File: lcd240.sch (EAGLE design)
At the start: 27 parts, among them IC1 CAT4238TD-GT3

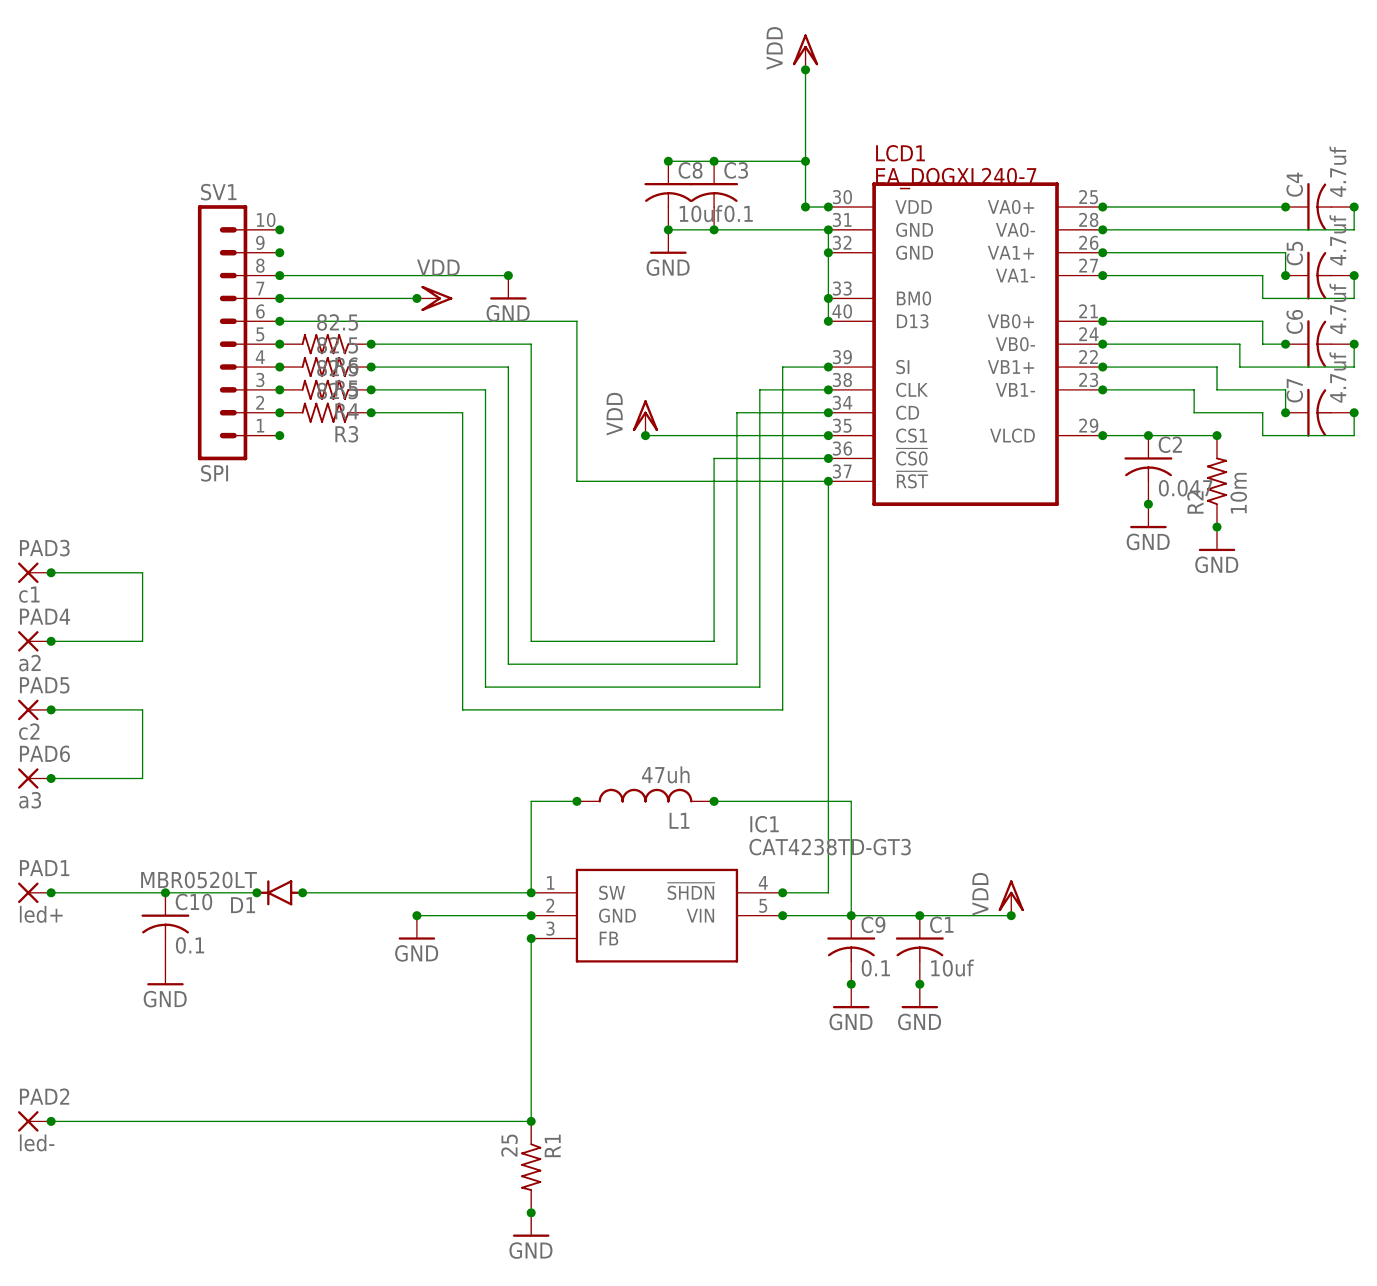
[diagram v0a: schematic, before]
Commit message: up
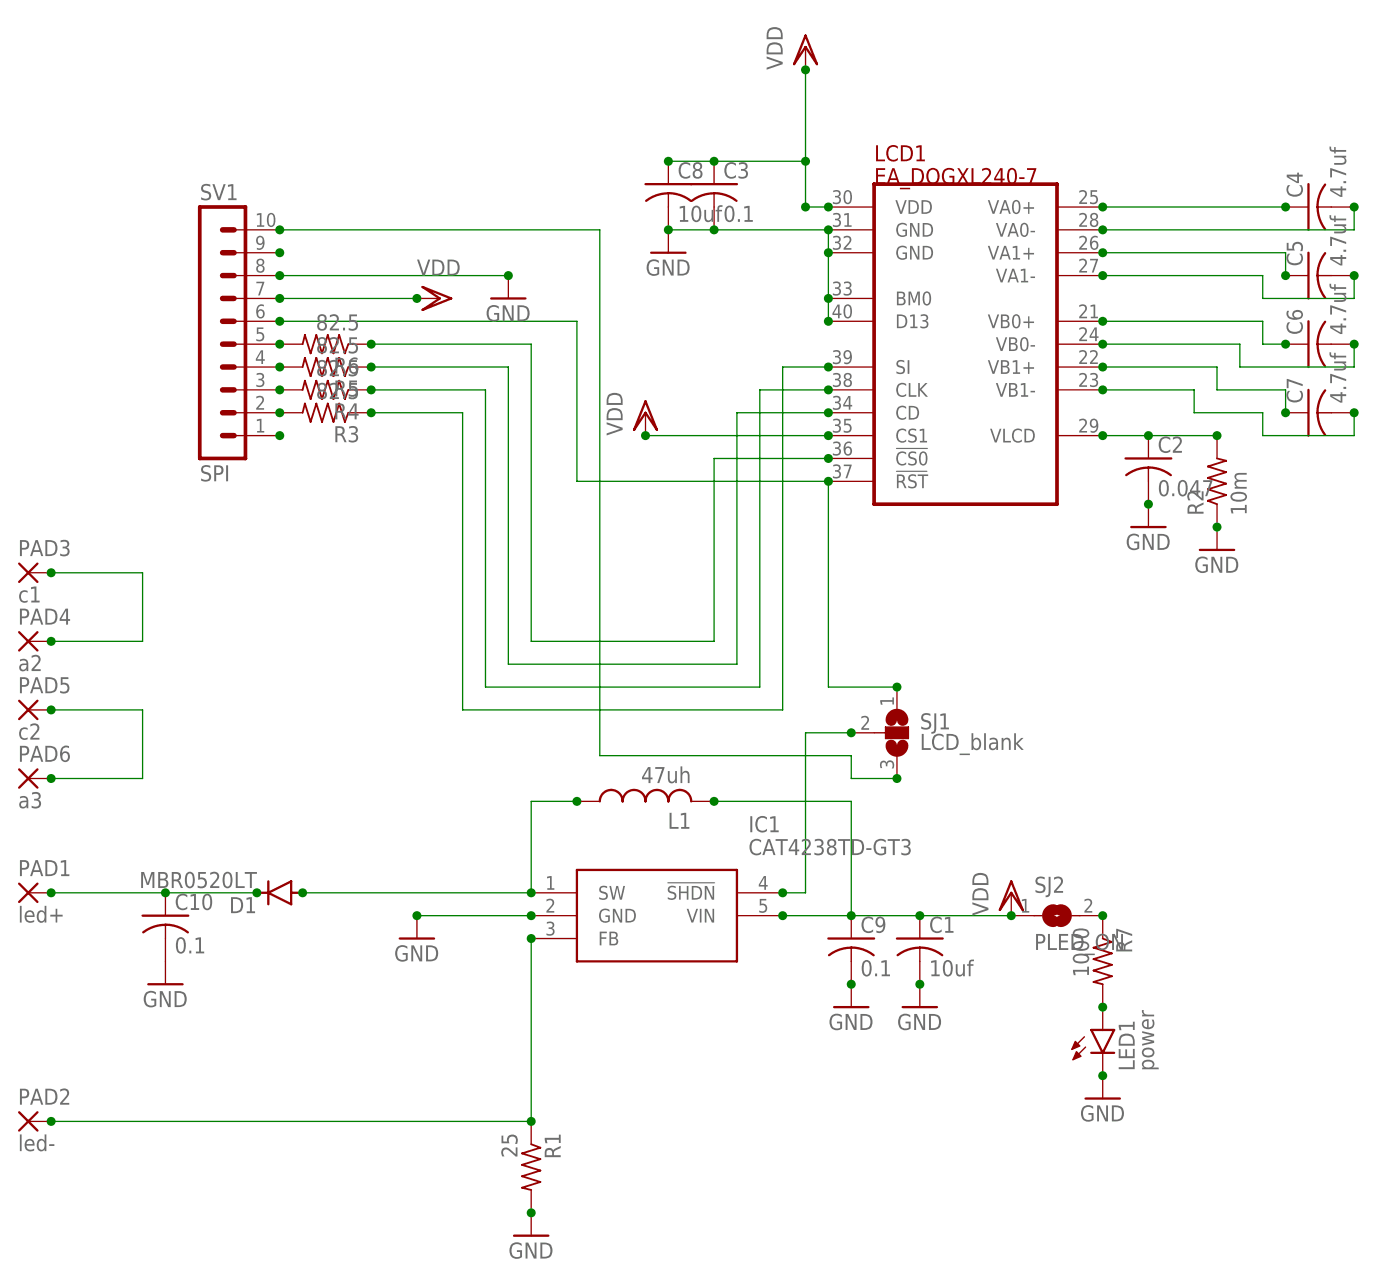
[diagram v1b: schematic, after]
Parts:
- added LED1: power, led:LEDSML0805
- added R7: 1000, rcl:R-US_R0805
- added SJ1: LCD_blank, jumper:SJ2W
- added SJ2: PLED_ON, jumper:SJ
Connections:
- new net N$27: IC1.!SHDN, SJ1.2
- new net N$28: R7.1, SJ2.2
- new net N$29: LED1.A, R7.2
- net GND: now also LED1.C
- net N$17: now also SJ1.3
- net N$4: now also SJ1.1; no longer IC1.!SHDN
- net VDD: now also SJ2.1
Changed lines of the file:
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@@
 <class number="1" name="icurrent" width="0.3048" drill="0">
 </class>
-<class number="2" name="led" width="0.508" drill="0">
+<class number="2" name="led" width="0.3048" drill="0">
 <clearance class="2" value="0.4064"/>
 </class>
@@
 <part name="PAD5" library="wirepad" library_urn="urn:adsk.eagle:library:412" deviceset="1,6/0,8" device="" package3d_urn="urn:adsk.eagle:package:30830/1" value="c2"/>
 <part name="PAD6" library="wirepad" library_urn="urn:adsk.eagle:library:412" deviceset="1,6/0,8" device="" package3d_urn="urn:adsk.eagle:package:30830/1" value="a3"/>
+<part name="SJ1" library="jumper" library_urn="urn:adsk.eagle:library:252" deviceset="SJ2W" device="" package3d_urn="urn:adsk.eagle:package:15474/1" value="LCD_blank"/>
+<part name="SJ2" library="jumper" library_urn="urn:adsk.eagle:library:252" deviceset="SJ" device="" package3d_urn="urn:adsk.eagle:package:15471/1" value="PLED_ON"/>
+<part name="R7" library="rcl" library_urn="urn:adsk.eagle:library:334" deviceset="R-US_" device="R0805" package3d_urn="urn:adsk.eagle:package:23553/2" value="1000"/>
+<part name="LED1" library="led" library_urn="urn:adsk.eagle:library:259" deviceset="LED" device="SML0805" package3d_urn="urn:adsk.eagle:package:15830/1" value="power"/>
+<part name="GND10" library="supply1" library_urn="urn:adsk.eagle:library:371" deviceset="GND" device=""/>
 </parts>
 <sheets>
@@
 <attribute name="NAME" x="-34.163" y="-5.7658" size="1.778" layer="95"/>
 <attribute name="VALUE" x="-34.163" y="-10.922" size="1.778" layer="96"/>
+</instance>
+<instance part="SJ1" gate="G$1" x="63.5" y="-2.54" smashed="yes">
+<attribute name="NAME" x="66.04" y="-2.159" size="1.778" layer="95"/>
+<attribute name="VALUE" x="66.04" y="-4.445" size="1.778" layer="96"/>
+</instance>
+<instance part="SJ2" gate="1" x="81.28" y="-22.86" smashed="yes">
+<attribute name="NAME" x="78.74" y="-20.32" size="1.778" layer="95"/>
+<attribute name="VALUE" x="78.74" y="-26.67" size="1.778" layer="96"/>
+</instance>
+<instance part="R7" gate="G$1" x="86.36" y="-27.94" smashed="yes" rot="R270">
+<attribute name="NAME" x="87.8586" y="-24.13" size="1.778" layer="95" rot="R270"/>
+<attribute name="VALUE" x="83.058" y="-24.13" size="1.778" layer="96" rot="R270"/>
+</instance>
+<instance part="LED1" gate="G$1" x="86.36" y="-35.56" smashed="yes">
+<attribute name="NAME" x="89.916" y="-40.132" size="1.778" layer="95" rot="R90"/>
+<attribute name="VALUE" x="92.075" y="-40.132" size="1.778" layer="96" rot="R90"/>
+</instance>
+<instance part="GND10" gate="1" x="86.36" y="-43.18" smashed="yes">
+<attribute name="VALUE" x="83.82" y="-45.72" size="1.778" layer="96"/>
 </instance>
 </instances>
@@
 <junction x="43.18" y="-10.16"/>
 <junction x="76.2" y="-22.86"/>
+<pinref part="SJ2" gate="1" pin="1"/>
 </segment>
 </net>
@@
 <pinref part="GND9" gate="1" pin="GND"/>
 </segment>
+<segment>
+<pinref part="LED1" gate="G$1" pin="C"/>
+<pinref part="GND10" gate="1" pin="GND"/>
+<junction x="86.36" y="-40.64"/>
+</segment>
 </net>
 <net name="N$3" class="0">
@@
 <pinref part="LCD1" gate="G$1" pin="!RST!"/>
 <wire x1="55.88" y1="25.4" x2="27.94" y2="25.4" width="0.1524" layer="91"/>
-<junction x="55.88" y="25.4"/>
 <pinref part="SV1" gate="1" pin="6"/>
 <junction x="-5.08" y="43.18"/>
 <wire x1="-5.08" y1="43.18" x2="27.94" y2="43.18" width="0.1524" layer="91"/>
 <wire x1="27.94" y1="43.18" x2="27.94" y2="25.4" width="0.1524" layer="91"/>
-<pinref part="IC1" gate="G$1" pin="!SHDN"/>
-<wire x1="50.8" y1="-20.32" x2="55.88" y2="-20.32" width="0.1524" layer="91"/>
-<wire x1="55.88" y1="-20.32" x2="55.88" y2="25.4" width="0.1524" layer="91"/>
-<junction x="50.8" y="-20.32"/>
+<pinref part="SJ1" gate="G$1" pin="1"/>
+<wire x1="55.88" y1="25.4" x2="55.88" y2="2.54" width="0.1524" layer="91"/>
+<wire x1="55.88" y1="2.54" x2="63.5" y2="2.54" width="0.1524" layer="91"/>
+<junction x="63.5" y="2.54"/>
+<junction x="55.88" y="25.4"/>
 </segment>
 </net>
@@
 <pinref part="SV1" gate="1" pin="10"/>
 <junction x="-5.08" y="53.34"/>
+<wire x1="-5.08" y1="53.34" x2="30.48" y2="53.34" width="0.1524" layer="91"/>
+<wire x1="30.48" y1="53.34" x2="30.48" y2="-5.08" width="0.1524" layer="91"/>
+<wire x1="30.48" y1="-5.08" x2="58.42" y2="-5.08" width="0.1524" layer="91"/>
+<wire x1="58.42" y1="-5.08" x2="58.42" y2="-7.62" width="0.1524" layer="91"/>
+<pinref part="SJ1" gate="G$1" pin="3"/>
+<wire x1="58.42" y1="-7.62" x2="63.5" y2="-7.62" width="0.1524" layer="91"/>
+<junction x="63.5" y="-7.62"/>
 </segment>
 </net>
@@
 </segment>
 </net>
+<net name="N$27" class="0">
+<segment>
+<pinref part="SJ1" gate="G$1" pin="2"/>
+<wire x1="58.42" y1="-2.54" x2="53.34" y2="-2.54" width="0.1524" layer="91"/>
+<wire x1="53.34" y1="-2.54" x2="53.34" y2="-20.32" width="0.1524" layer="91"/>
+<pinref part="IC1" gate="G$1" pin="!SHDN"/>
+<wire x1="53.34" y1="-20.32" x2="50.8" y2="-20.32" width="0.1524" layer="91"/>
+<junction x="58.42" y="-2.54"/>
+<junction x="50.8" y="-20.32"/>
+</segment>
+</net>
+<net name="N$28" class="0">
+<segment>
+<pinref part="SJ2" gate="1" pin="2"/>
+<pinref part="R7" gate="G$1" pin="1"/>
+<junction x="86.36" y="-22.86"/>
+</segment>
+</net>
+<net name="N$29" class="0">
+<segment>
+<pinref part="R7" gate="G$1" pin="2"/>
+<pinref part="LED1" gate="G$1" pin="A"/>
+<junction x="86.36" y="-33.02"/>
+</segment>
+</net>
